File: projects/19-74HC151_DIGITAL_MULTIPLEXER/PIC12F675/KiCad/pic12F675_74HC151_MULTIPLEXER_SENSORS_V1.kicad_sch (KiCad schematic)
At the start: 9 parts, among them U1 PIC12F675-IP, U2 74151, U3 ZMCT103C, U4 ZMCT103C, U5 ZMCT103C, U6 ZMCT103C

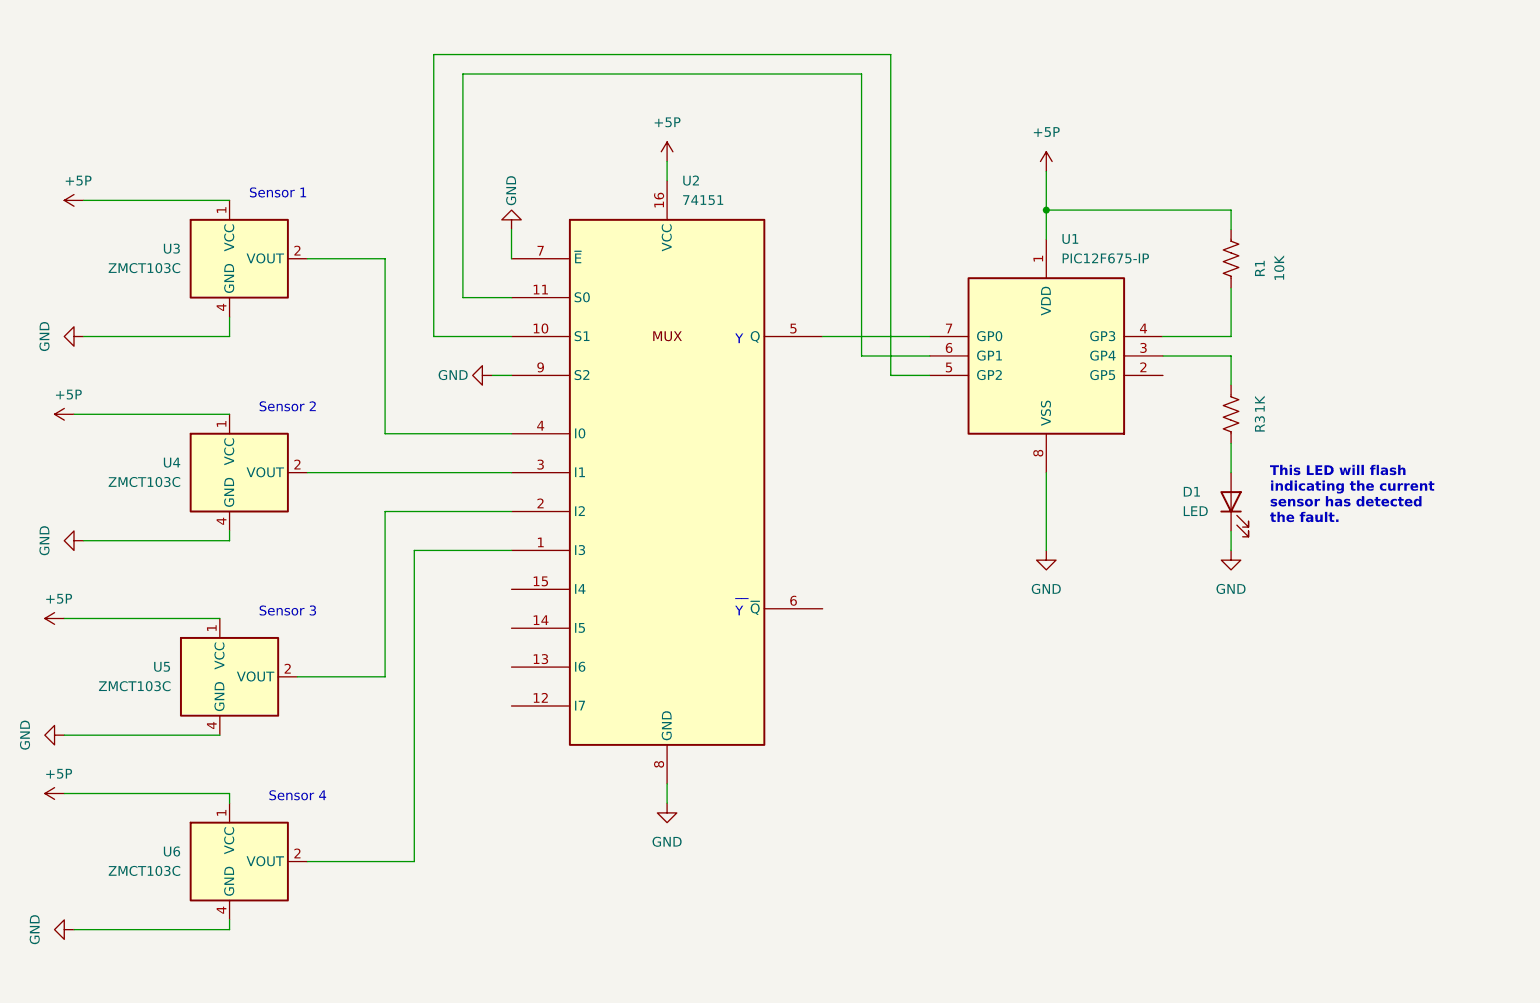
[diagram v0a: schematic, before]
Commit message: Doc
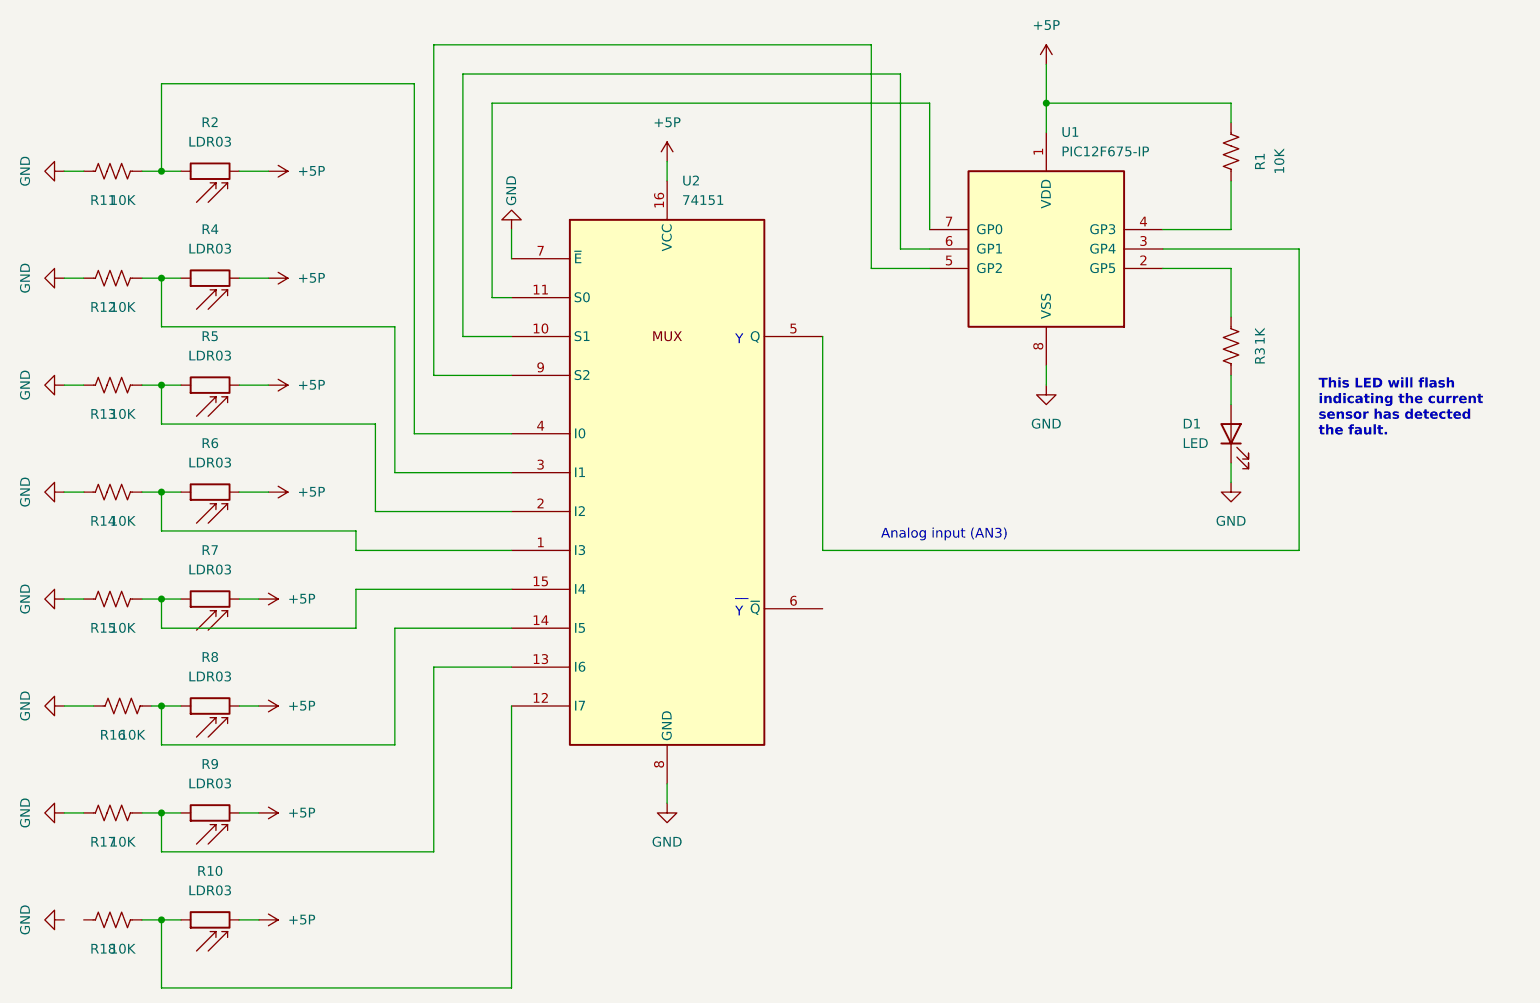
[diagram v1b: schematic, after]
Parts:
- removed U3, U4, U5, U6: ZMCT103C, Sensor_Current:Allegro_SIP-4, symbol Sensor_Current:A1363xKTTN-1
- added R10, R2, R4, R5, R6, R7, R8, R9: LDR03, OptoDevice:R_LDR_10x8.5mm_P7.6mm_Vertical, symbol Sensor_Optical:LDR03
- added R11, R12, R13, R14, R15, R16, R17, R18: 10K, symbol Device:R_US
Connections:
- net +5P: now also R10.2, R2.2, R4.2, R5.2, R6.2, R7.2, R8.2, R9.2
- net GND: now also R11.2, R12.2, R13.2, R14.2, R15.2, R16.2, R17.2; no longer U2.9 (S2)
- net at U2.1 (I3): now also R14.1, R6.1
- net at U2.2 (I2): now also R13.1, R5.1
- net at U2.3 (I1): now also R12.1, R4.1
- net at U2.10 (S1): now also U1.6 (GP1); no longer U1.5 (GP2)
- net at U2.11 (S0): now also U1.7 (GP0); no longer U1.6 (GP1)
- net at U2.12 (I7): now also R10.1, R18.1
- net at U2.13 (I6): now also R17.1, R9.1
- net at U2.14 (I5): now also R16.1, R8.1
- net at U2.15 (I4): now also R15.1, R7.1
- net at U2.4 (I0): now also R11.1, R2.1
- net at U2.5 (Q): now also U1.3 (GP4); no longer U1.7 (GP0)
- net at U1.2 (GP5): now also R3.1
- new net: U1.5 (GP2), U2.9 (S2)
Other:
- note added: "Analog input (AN3)"
- note removed: "Sensor 1"
- note removed: "Sensor 2"
- note removed: "Sensor 3"
- note removed: "Sensor 4"
- title: PIC12F675 and 74HC151 monitoring 4 sensors -> PIC12F675 and 74HC151 monitoring 8 sensors
- moved on the sheet: D1, R1, R3, U1
